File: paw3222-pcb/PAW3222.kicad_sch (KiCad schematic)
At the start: 7 parts, among them J1 Conn_01x06_Socket, U1 PAW3220LU

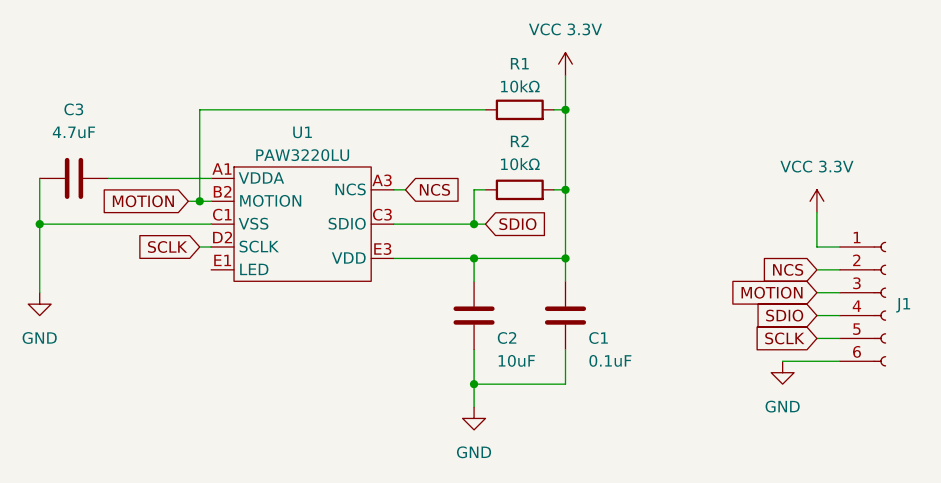
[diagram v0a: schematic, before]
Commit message: add led
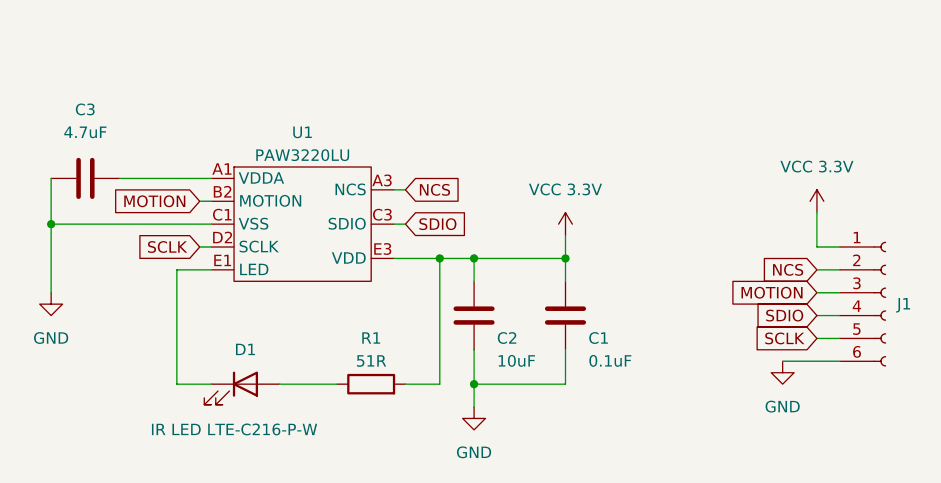
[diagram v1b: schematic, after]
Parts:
- removed R2: 10kΩ, Resistor_SMD:R_0603_1608Metric, symbol Device:R
- added D1: IR LED LTE-C216-P-W, paw3222:LTE-C216-P-W, symbol Device:LED
- C1, C2, C3: footprint Capacitor_SMD:C_0603_1608Metric -> Capacitor_SMD:C_0402_1005Metric
- R1: value 10kΩ -> 51R; footprint Resistor_SMD:R_0603_1608Metric -> Resistor_SMD:R_0402_1005Metric
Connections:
- net MOTION: no longer R1.1
- net at U1.E1 (LED): now also D1.1 (K)
- new net: D1.2 (A), R1.1
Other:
- moved on the sheet: C3
